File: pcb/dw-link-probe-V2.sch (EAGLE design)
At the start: 27 parts, among them IC1 74LVC1G125DBV, IC2 74LVC1G125DBV, IC3 74LVC1G125DBV, IC4 TS1117BCW33_RPG, Q1 BSS138, Q2 IRLML6402, Q3 IRLML6402

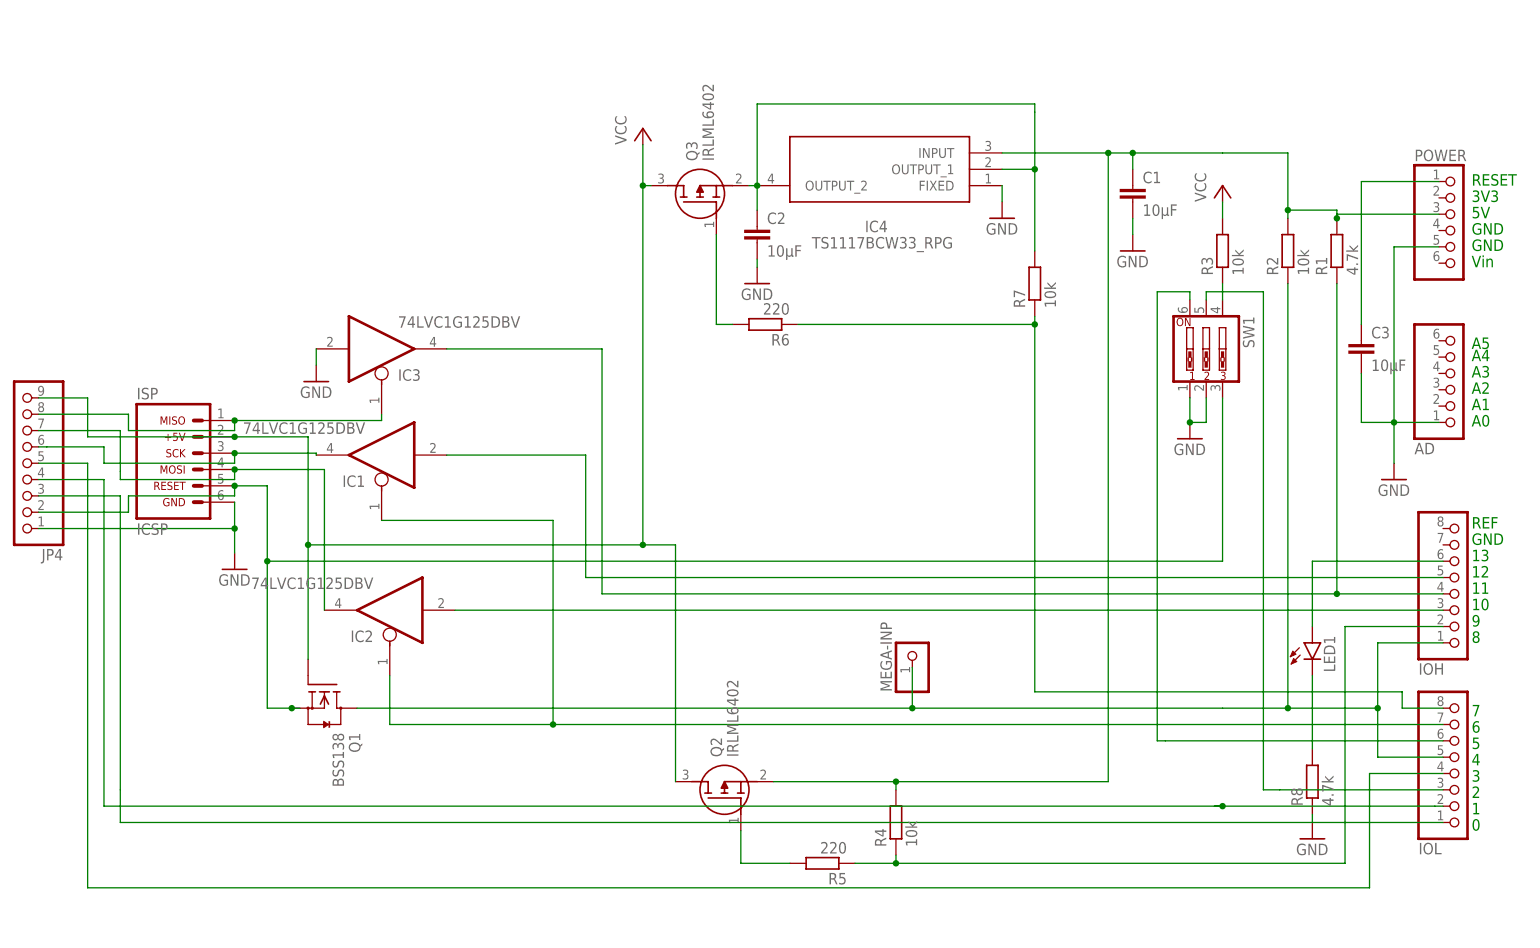
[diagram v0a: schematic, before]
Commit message: changelog ficed
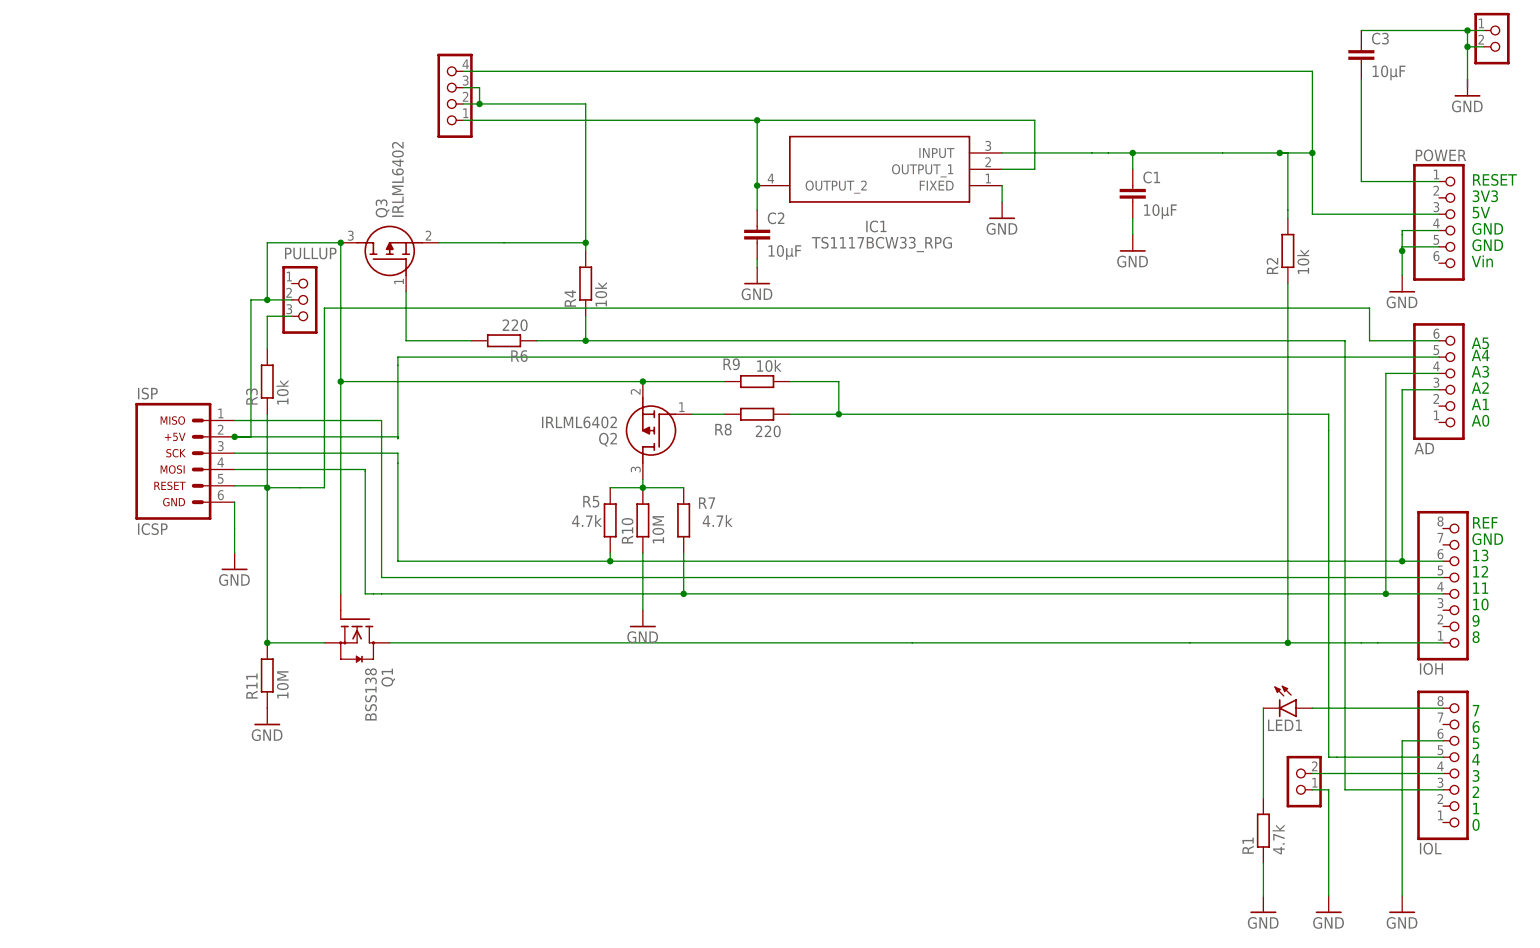
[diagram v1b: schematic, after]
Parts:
- removed IC2, IC3: 74LVC1G125DBV, 74xx-little-us:74LVC1G125DBV
- removed IC4: TS1117BCW33_RPG, TS1117BCW33_RPG:TS1117BCW33_RPG
- removed JP4: (no value), pinhead:PINHD-1X9
- removed MEGA-INP: (no value), pinhead:PINHD-1X1
- removed SW1: (no value), special:SW_DIP-3
- added DEBUG, RES_EN: CON_HEADER_1X02-PTH, dp_devices:CON_HEADER_1X02-PTH
- added PULLUP: CON_HEADER_1X03-PTH, dp_devices:CON_HEADER_1X03-PTH
- added R10, R11: 10M, rcl:R-EU_R1206
- added R9: 10k, rcl:R-EU_R1206
- added SUPPLY: CON_HEADER_1X04, dp_devices:CON_HEADER_1X04
- IC1: value 74LVC1G125DBV -> TS1117BCW33_RPG; device 74xx-little-us:74LVC1G125DBV -> TS1117BCW33_RPG:TS1117BCW33_RPG
- R5: value 220 -> 4.7k
- R7: value 10k -> 4.7k
- R8: value 4.7k -> 220
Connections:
- removed net N$20: IOL.2, JP4.4
- removed net N$21: IOH.6, LED1.A
- removed net N$23: IOL.1, JP4.3
- removed net N$24: IOL.4, JP4.5
- removed net N$5 (its old number): IC2A.O, ISP.4, JP4.7
- removed net N$7: IC2A.I, IOH.3
- removed net VCC: ISP.2, JP4.9, Q1.G, Q2.D, Q3.D, R3.2
- new net N$17: IOL.5, R8.1, R9.1
- net GND: now also C3.1, DEBUG.1, IC1.FIXED, IOL.6, POWER.4, R1.1, R10.1, R11.1, RES_EN.1, RES_EN.2; no longer AD.1, C3.2, IC3A.I, IC4.FIXED, JP4.1, R8.1, SW1.1, SW1.2
- net N$1: now also IC1.INPUT, SUPPLY.4; no longer IC4.INPUT, Q2.S, R1.2, R4.2
- net N$10: now also PULLUP.3, R3.2; no longer Q2.G, R5.2
- net N$11: now also IOH.5, ISP.1; no longer ISP.5, JP4.2, Q1.S, SW1.3
- net N$12: now also AD.3, IOH.6, ISP.3, R5.1; no longer R3.1, SW1.4
- net N$13: now also AD.4, IOH.4, ISP.4, R7.1; no longer IOL.6, SW1.6
- net N$14: now also Q3.S, R4.2, SUPPLY.2, SUPPLY.3; no longer IOL.3, SW1.5
- net N$15: now also IC1.OUTPUT_1, IC1.OUTPUT_2, SUPPLY.1; no longer IC4.OUTPUT_1, IC4.OUTPUT_2, Q3.S, R7.2
- net N$16: now also Q2.D, R10.2, R5.2, R7.2; no longer IOH.2, R4.1, R5.1
- net N$18: now also DEBUG.2, IOL.4; no longer IOL.8, R6.1, R7.1
- net N$19: now also C3.2; no longer C3.1
- net N$2: no longer IOL.5, MEGA-INP.1
- net N$22: now also R1.2; no longer R8.2
- net N$3: now also AD.6, ISP.5, Q1.S, R11.2, R3.1; no longer IC1A.O, ISP.3, JP4.6
- net N$4: now also IOL.3, R4.1, R6.1; no longer IC3A.OE, ISP.1, JP4.8
- net N$6: now also AD.5, ISP.2, PULLUP.2, Q1.G, Q2.S, Q3.D, R9.2; no longer IC1A.OE, IC2A.OE, IOL.7
- net N$8: now also Q2.G, R8.2; no longer IC1A.I, IOH.5
- net N$9: now also IOL.8, LED1.A; no longer IC3A.O, IOH.4, R1.1
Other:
- moved on the sheet: C3, LED1, Q1, Q2, Q3, R1, R3, R4, R5, R6, R7, R8

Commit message: pcb fix
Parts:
- renumbered RES_EN to RESDIS
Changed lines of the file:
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@@
 <setting verticaltext="up"/>
 </settings>
-<grid distance="0.05" unitdist="inch" unit="inch" style="lines" multiple="1" display="no" altdistance="0.01" altunitdist="inch" altunit="inch"/>
+<grid distance="0.1" unitdist="inch" unit="inch" style="lines" multiple="1" display="no" altdistance="0.01" altunitdist="inch" altunit="inch"/>
 <layers>
 <layer number="1" name="Top" color="4" fill="1" visible="no" active="no"/>
@@
 <part name="R9" library="rcl" library_urn="urn:adsk.eagle:library:334" deviceset="R-EU_" device="R1206" package3d_urn="urn:adsk.eagle:package:23540/2" value="10k"/>
 <part name="DEBUG" library="dp_devices" deviceset="CON_HEADER_1X02" device="-PTH"/>
-<part name="RES_EN" library="dp_devices" deviceset="CON_HEADER_1X02" device="-PTH"/>
+<part name="RESDIS" library="dp_devices" deviceset="CON_HEADER_1X02" device="-PTH"/>
 <part name="GND3" library="supply1" library_urn="urn:adsk.eagle:library:371" deviceset="GND" device=""/>
 <part name="GND1" library="supply1" library_urn="urn:adsk.eagle:library:371" deviceset="GND" device=""/>
@@
 <sheet>
 <plain>
-<text x="215.265" y="21.59" size="1.778" layer="91" grouprefs="PINS IOL1 IO">0</text>
-<text x="215.265" y="24.13" size="1.778" layer="91" grouprefs="PINS IOL1 IO">1</text>
-<text x="215.265" y="26.67" size="1.778" layer="91" grouprefs="PINS IOL1 IO">2</text>
-<text x="215.265" y="29.21" size="1.778" layer="91" grouprefs="PINS IOL1 IO">3</text>
-<text x="215.265" y="31.75" size="1.778" layer="91" grouprefs="PINS IOL1 IO">4</text>
-<text x="215.265" y="34.29" size="1.778" layer="91" grouprefs="PINS IOL1 IO">5</text>
-<text x="215.265" y="36.83" size="1.778" layer="91" grouprefs="PINS IOL1 IO">6</text>
-<text x="215.265" y="39.37" size="1.778" layer="91" grouprefs="PINS IOL1 IO">7</text>
-<text x="215.265" y="50.8" size="1.778" layer="91" grouprefs="PINS LABH IO">8</text>
-<text x="215.265" y="53.34" size="1.778" layer="91" grouprefs="PINS LABH IO">9</text>
-<text x="215.265" y="55.88" size="1.778" layer="91" grouprefs="PINS LABH IO">10</text>
-<text x="215.265" y="58.42" size="1.778" layer="91" grouprefs="PINS IO">11</text>
-<text x="215.265" y="60.96" size="1.778" layer="91" grouprefs="PINS LABH IO">12</text>
-<text x="215.265" y="63.5" size="1.778" layer="91" grouprefs="PINS LABH IO">13</text>
-<text x="215.265" y="66.04" size="1.778" layer="91" grouprefs="PINS IO">GND</text>
-<text x="215.265" y="68.58" size="1.778" layer="91" grouprefs="PINS IO">REF</text>
-<text x="215.265" y="121.92" size="1.778" layer="91" grouprefs="PINS IO">RESET</text>
-<text x="215.265" y="119.38" size="1.778" layer="91" grouprefs="PINS IO">3V3</text>
-<text x="215.265" y="116.84" size="1.778" layer="91" grouprefs="PINS IO">5V</text>
-<text x="215.265" y="114.3" size="1.778" layer="91" grouprefs="PINS IO">GND</text>
-<text x="215.265" y="111.76" size="1.778" layer="91" grouprefs="PINS IO">GND</text>
-<text x="215.265" y="109.22" size="1.778" layer="91" grouprefs="PINS IO">Vin</text>
-<text x="215.265" y="96.52" size="1.778" layer="91" grouprefs="PINS IO">A5</text>
-<text x="215.265" y="94.615" size="1.778" layer="91" grouprefs="PINS IO">A4</text>
-<text x="215.265" y="92.075" size="1.778" layer="91" grouprefs="PINS IO">A3</text>
-<text x="215.265" y="89.535" size="1.778" layer="91" grouprefs="PINS IO">A2</text>
-<text x="215.265" y="86.995" size="1.778" layer="91" grouprefs="PINS IO">A1</text>
-<text x="215.265" y="84.455" size="1.778" layer="91" grouprefs="PINS IO">A0</text>
+<text x="215.265" y="21.59" size="1.778" layer="91" grouprefs="IO IOL1 PINS">0</text>
+<text x="215.265" y="24.13" size="1.778" layer="91" grouprefs="IO IOL1 PINS">1</text>
+<text x="215.265" y="26.67" size="1.778" layer="91" grouprefs="IO IOL1 PINS">2</text>
+<text x="215.265" y="29.21" size="1.778" layer="91" grouprefs="IO IOL1 PINS">3</text>
+<text x="215.265" y="31.75" size="1.778" layer="91" grouprefs="IO IOL1 PINS">4</text>
+<text x="215.265" y="34.29" size="1.778" layer="91" grouprefs="IO IOL1 PINS">5</text>
+<text x="215.265" y="36.83" size="1.778" layer="91" grouprefs="IO IOL1 PINS">6</text>
+<text x="215.265" y="39.37" size="1.778" layer="91" grouprefs="IO IOL1 PINS">7</text>
+<text x="215.265" y="50.8" size="1.778" layer="91" grouprefs="IO LABH PINS">8</text>
+<text x="215.265" y="53.34" size="1.778" layer="91" grouprefs="IO LABH PINS">9</text>
+<text x="215.265" y="55.88" size="1.778" layer="91" grouprefs="IO LABH PINS">10</text>
+<text x="215.265" y="58.42" size="1.778" layer="91" grouprefs="IO PINS">11</text>
+<text x="215.265" y="60.96" size="1.778" layer="91" grouprefs="IO LABH PINS">12</text>
+<text x="215.265" y="63.5" size="1.778" layer="91" grouprefs="IO LABH PINS">13</text>
+<text x="215.265" y="66.04" size="1.778" layer="91" grouprefs="IO PINS">GND</text>
+<text x="215.265" y="68.58" size="1.778" layer="91" grouprefs="IO PINS">REF</text>
+<text x="215.265" y="121.92" size="1.778" layer="91" grouprefs="IO PINS">RESET</text>
+<text x="215.265" y="119.38" size="1.778" layer="91" grouprefs="IO PINS">3V3</text>
+<text x="215.265" y="116.84" size="1.778" layer="91" grouprefs="IO PINS">5V</text>
+<text x="215.265" y="114.3" size="1.778" layer="91" grouprefs="IO PINS">GND</text>
+<text x="215.265" y="111.76" size="1.778" layer="91" grouprefs="IO PINS">GND</text>
+<text x="215.265" y="109.22" size="1.778" layer="91" grouprefs="IO PINS">Vin</text>
+<text x="215.265" y="96.52" size="1.778" layer="91" grouprefs="IO PINS">A5</text>
+<text x="215.265" y="94.615" size="1.778" layer="91" grouprefs="IO PINS">A4</text>
+<text x="215.265" y="92.075" size="1.778" layer="91" grouprefs="IO PINS">A3</text>
+<text x="215.265" y="89.535" size="1.778" layer="91" grouprefs="IO PINS">A2</text>
+<text x="215.265" y="86.995" size="1.778" layer="91" grouprefs="IO PINS">A1</text>
+<text x="215.265" y="84.455" size="1.778" layer="91" grouprefs="IO PINS">A0</text>
 </plain>
 <instances>
-<instance part="IOL" gate="A" x="213.36" y="33.02" smashed="yes" rot="MR180" grouprefs="PINS IOL1 IO">
+<instance part="IOL" gate="A" x="213.36" y="33.02" smashed="yes" rot="MR180" grouprefs="IO IOL1 PINS">
 <attribute name="NAME" x="207.01" y="19.685" size="1.778" layer="95" rot="MR180"/>
 <attribute name="VALUE" x="207.01" y="45.72" size="1.778" layer="96" rot="MR180"/>
 </instance>
-<instance part="IOH" gate="A" x="213.36" y="60.96" smashed="yes" rot="MR180" grouprefs="PINS IO">
+<instance part="IOH" gate="A" x="213.36" y="60.96" smashed="yes" rot="MR180" grouprefs="IO PINS">
 <attribute name="NAME" x="207.01" y="47.625" size="1.778" layer="95" rot="MR180"/>
 <attribute name="VALUE" x="207.01" y="73.66" size="1.778" layer="96" rot="MR180"/>
 </instance>
-<instance part="AD" gate="A" x="212.725" y="92.71" smashed="yes" rot="MR180" grouprefs="PINS IO">
+<instance part="AD" gate="A" x="212.725" y="92.71" smashed="yes" rot="MR180" grouprefs="IO PINS">
 <attribute name="NAME" x="206.375" y="81.915" size="1.778" layer="95" rot="MR180"/>
 <attribute name="VALUE" x="206.375" y="102.87" size="1.778" layer="96" rot="MR180"/>
 </instance>
-<instance part="POWER" gate="A" x="212.725" y="114.935" smashed="yes" grouprefs="PINS IO">
+<instance part="POWER" gate="A" x="212.725" y="114.935" smashed="yes" grouprefs="IO PINS">
 <attribute name="NAME" x="206.375" y="125.73" size="1.778" layer="95"/>
 <attribute name="VALUE" x="206.375" y="104.775" size="1.778" layer="96"/>
@@
 </instance>
 <instance part="DEBUG" gate="J" x="190.5" y="27.94" smashed="yes" rot="R180"/>
-<instance part="RES_EN" gate="J" x="217.17" y="146.05" smashed="yes"/>
+<instance part="RESDIS" gate="J" x="217.17" y="146.05" smashed="yes"/>
 <instance part="GND3" gate="1" x="193.04" y="8.89" smashed="yes">
 <attribute name="VALUE" x="190.5" y="6.35" size="1.778" layer="96"/>
@@
 <segment>
 <pinref part="GND8" gate="1" pin="GND"/>
-<pinref part="RES_EN" gate="J" pin="2"/>
+<pinref part="RESDIS" gate="J" pin="2"/>
 <wire x1="217.17" y1="143.51" x2="214.63" y2="143.51" width="0.1524" layer="91"/>
 <wire x1="214.63" y1="143.51" x2="214.63" y2="138.43" width="0.1524" layer="91"/>
 <wire x1="214.63" y1="138.43" x2="214.63" y2="137.16" width="0.1524" layer="91"/>
 <pinref part="C3" gate="G$1" pin="1"/>
-<pinref part="RES_EN" gate="J" pin="1"/>
+<pinref part="RESDIS" gate="J" pin="1"/>
 <wire x1="198.12" y1="146.05" x2="214.63" y2="146.05" width="0.1524" layer="91"/>
 <wire x1="214.63" y1="146.05" x2="217.17" y2="146.05" width="0.1524" layer="91"/>
